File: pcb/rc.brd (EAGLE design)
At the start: 40.6 x 58.4 mm, 61 parts, among them IC2 TP4056

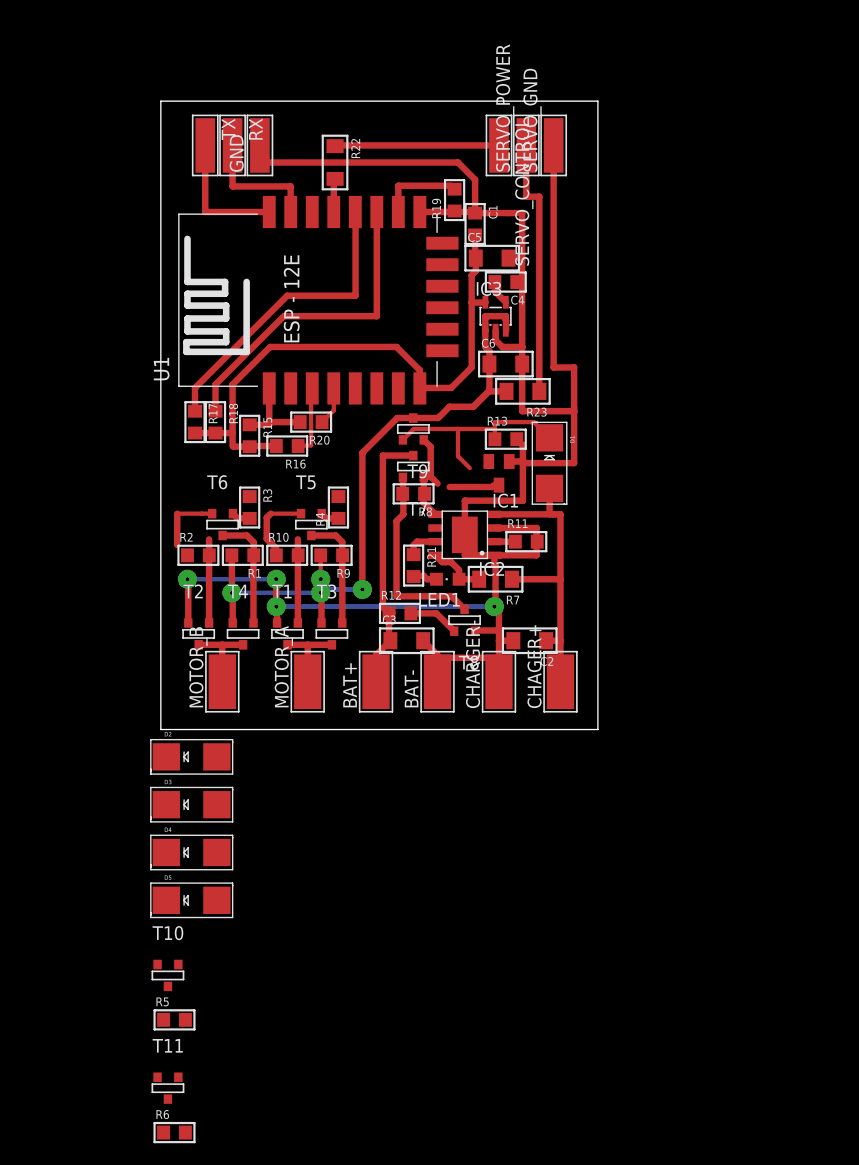
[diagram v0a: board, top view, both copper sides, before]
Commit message: begin pcb v2
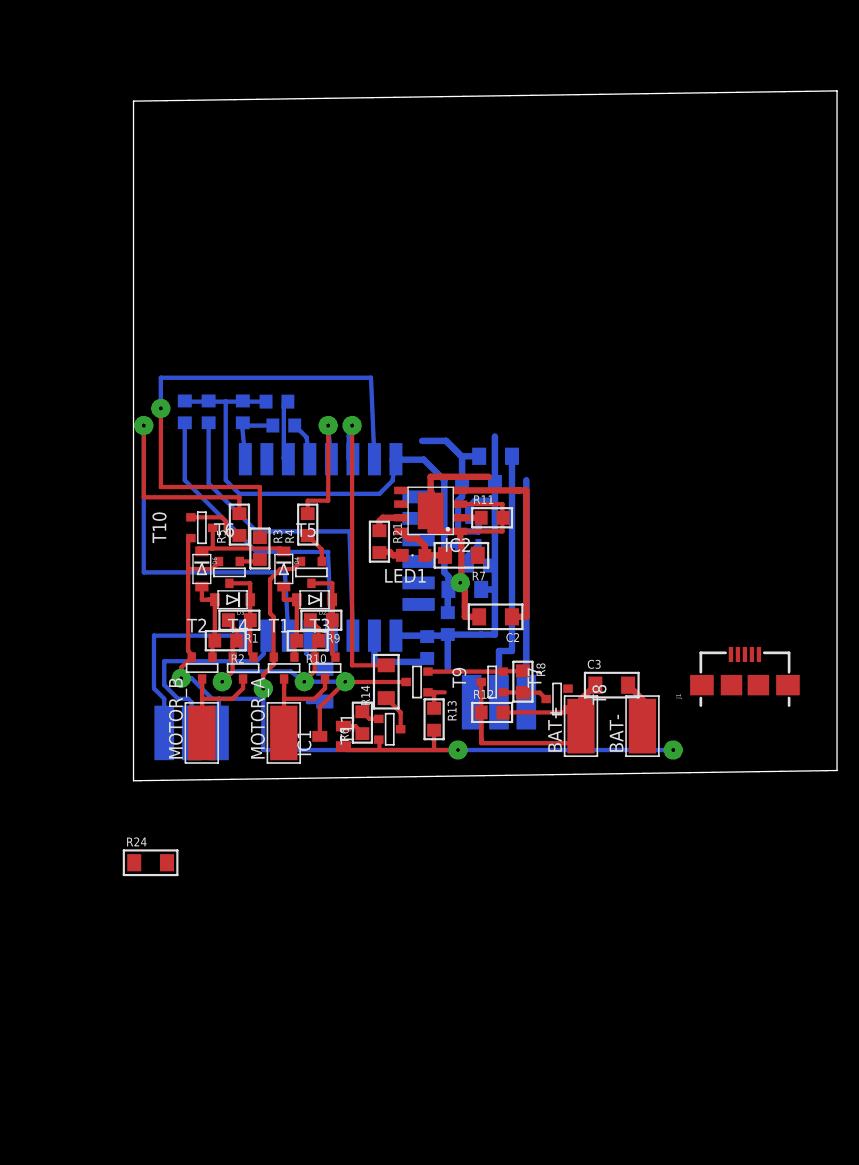
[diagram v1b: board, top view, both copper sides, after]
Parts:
- removed CHAGER+, CHARGER-: WIREPADSMD5-2,5, wirepad:5-2,5
- removed D1, D5: (no value), skydrop:SMADIODE
- added D6: (no value), skydrop:SOD-123FL
- added J1: (no value), skydrop:USB-AB-MICRO-SMD
- added R14: 0, skydrop:R1206
- added R24: (no value), skydrop:R1206
- D2, D3, D4: device skydrop:SMADIODE -> skydrop:SOD-123FL
- moved GND 54.7 mm to (5.40, 4.13), flipped to the bottom, turned to 180 degrees
- moved RX 54.7 mm to (2.86, 4.13), flipped to the bottom, turned to 0 degrees
- moved TX 54.7 mm to (0.32, 4.13), flipped to the bottom, turned to 0 degrees
- moved SERVO_CONTROL 51.8 mm to (28.9, 6.99), flipped to the bottom, turned to 0 degrees
- moved SERVO_GND 51.8 mm to (34.0, 6.99), flipped to the bottom, turned to 180 degrees
- moved SERVO_POWER 51.8 mm to (31.4, 6.99), flipped to the bottom, turned to 180 degrees
- moved R22 48.6 mm to (15.2, 8.57), flipped to the bottom, turned to 90 degrees
- moved R5 46.4 mm to (7.30, 23.5), turned to 90 degrees
- moved R6 41.9 mm to (18.7, 5.08), turned to 90 degrees
- moved T10 41.7 mm to (3.81, 23.2), turned to 90 degrees
- moved R19 41.7 mm to (24.8, 12.1), flipped to the bottom, turned to 270 degrees
- moved T11 39.2 mm to (21.3, 4.45), turned to 90 degrees
- moved C1 37.2 mm to (26.7, 14.3), flipped to the bottom, turned to 90 degrees
- moved C5 30.9 mm to (28.3, 17.5), flipped to the bottom, turned to 180 degrees
- moved IC1 29.0 mm to (15.9, 3.81), turned to 90 degrees
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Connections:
- net N$14 renamed BAT+
- net N$15 renamed TX
- net N$18 renamed RX
- removed net N$10: IC1.3, IC2.5, R8.1, T7.2, T9.2
- removed net N$24: D1.C, R13.1, T9.3
- new net BAT_CHRG: IC2.5, R8.1, T7.2, T9.2
- new net N$14: R14.1, T11.1
- net BAT_CHECK: now also R14.2; no longer T11.1
- net BAT_PROT: now also IC1.3
- net GND: now also J1.GND; no longer CHARGER-.1
- net N$31: now also D6.C; no longer D5.C
- net N$9: now also D6.A; no longer D5.A
- net V_CHRG: now also J1.VBUS, R13.1, R24.1, R24.2, T9.3; no longer CHAGER+.1, D1.A
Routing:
- net H_BCK: track 0.00 -> 51.2 mm, vias 0 -> 1
- net H_PWM: track 0.00 -> 49.7 mm, vias 0 -> 1
- net BAT_CHECK: track 0.00 -> 29.0 mm, vias 0 -> 1
- net N$24: track 20.4 -> 0.00 mm
- net N$12: track 19.1 -> 4.25 mm
- net GND: track 213.1 -> 198.3 mm, vias 4 -> 5
- net N$10: track 14.1 -> 0.00 mm
- net N$29: track 15.3 -> 1.59 mm
- net H_FWD: track 0.00 -> 13.3 mm, vias 0 -> 1
- net N$31: track 0.00 -> 10.4 mm
- net BAT_PROT: track 66.2 -> 56.8 mm, vias 4 -> 3
- net BAT_CHRG: track 0.00 -> 8.83 mm
- net RX: track 11.6 -> 19.9 mm
- net V_CHRG: track 30.5 -> 23.4 mm
- net TX: track 12.1 -> 17.9 mm
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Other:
- board size 40.6 x 58.4 mm -> 65.4 x 64.1 mm

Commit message: pcb
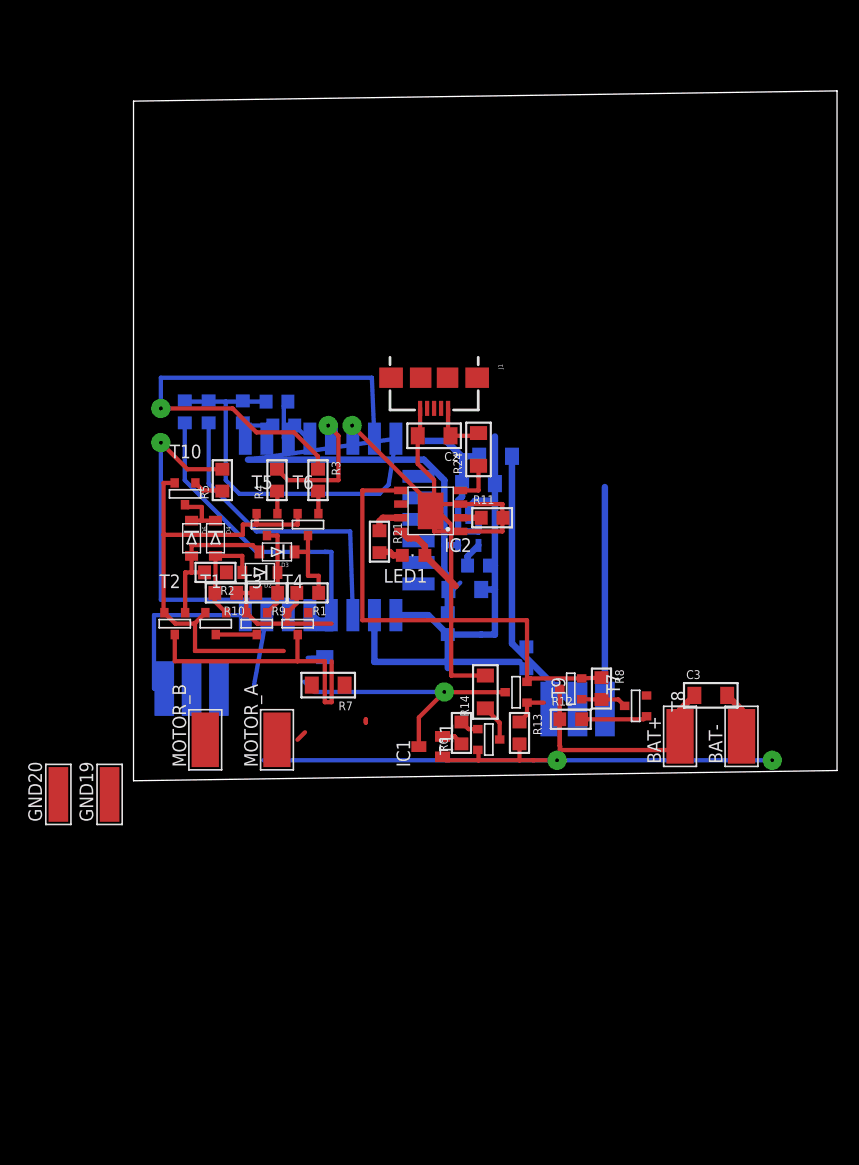
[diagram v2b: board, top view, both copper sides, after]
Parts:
- added GND19, GND20: WIREPADSMD5-1,8, wirepad:5-1,8
- R24: value (none) -> 0
- moved R24 49.0 mm to (29.5, 30.5), turned to 90 degrees
- moved J1 40.6 mm to (25.4, 37.1), turned to 270 degrees
- moved C2 17.8 mm to (25.4, 31.8)
- moved R7 17.3 mm to (15.6, 8.57)
- moved BAT- 9.26 mm to (54.0, 3.81)
- moved C3 9.26 mm to (51.1, 7.62)
- moved R14 9.26 mm to (30.2, 7.94)
- moved T9 9.26 mm to (33.0, 7.94)
- moved IC1 9.26 mm to (25.1, 2.86)
- moved R6 9.26 mm to (27.9, 4.13)
- moved T11 9.26 mm to (30.5, 3.49)
- moved BAT+ 9.26 mm to (48.3, 3.81)
- moved R19 9.26 mm to (34.0, 11.1)
- moved R10 8.82 mm to (6.03, 17.1)
- moved T6 8.55 mm to (13.7, 23.5)
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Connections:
- new net N$10: C2.1, J1.VBUS, R24.2
- net GND: now also GND20.1
- net N$21: now also GND19.1
- net V_CHRG: no longer C2.1, J1.VBUS, R24.2
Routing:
- net BAT_CHRG: track 8.83 -> 43.8 mm
- net VCC: track 53.3 -> 82.1 mm
- net N$4: track 11.0 -> 27.2 mm
- net V_CHRG: track 23.4 -> 7.64 mm
- net H_PWM: track 49.7 -> 34.6 mm
- net RX: track 19.9 -> 6.94 mm
- net N$26: track 7.72 -> 19.0 mm
- net N$33: track 11.0 -> 4.80 mm
- net N$9: track 8.65 -> 14.8 mm
- net N$10: track 0.00 -> 5.67 mm
- net H_BCK: track 51.2 -> 45.8 mm
- net N$31: track 10.4 -> 5.14 mm
- net N$32: track 5.77 -> 2.82 mm
- net BAT_PROT: track 56.8 -> 59.5 mm, vias 3 -> 1
- net BAT_CHECK: track 29.0 -> 31.5 mm
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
